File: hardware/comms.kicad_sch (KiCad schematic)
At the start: 8 parts, among them J5 USB_C_Receptacle_USB2.0, J6 CAN, J7 Conn_ARM_JTAG_SWD_10, U4 MCP2562-E-SN, U5 E73-2G4M08S1C

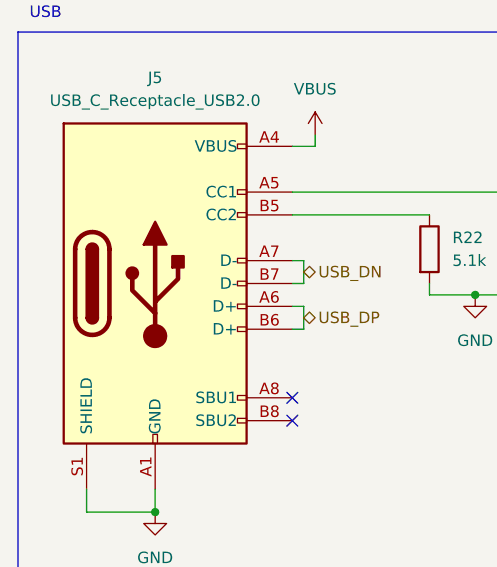
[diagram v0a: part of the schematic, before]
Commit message: Update design to KiCAD v7
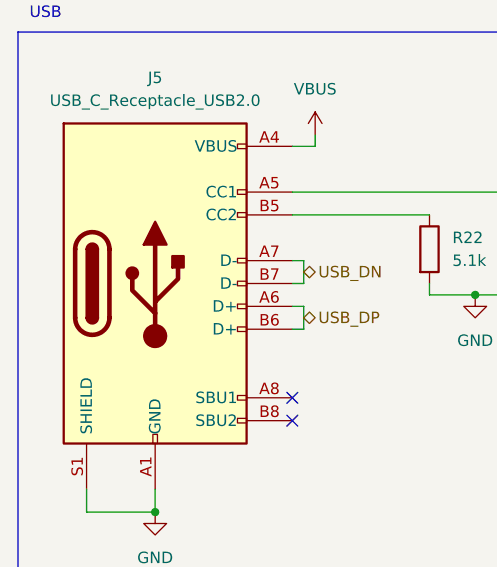
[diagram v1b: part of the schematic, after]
